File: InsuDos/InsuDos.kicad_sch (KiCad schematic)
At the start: 95 parts, among them J1 E-paper(C097), J2 USB_B_Micro, Q1 Si1308EDL, SW1 list, SW2 enter, SW3 dose, SW4 esc, U1 USBLC6-2P6, U2 TMP102xxDRL, U3 STNS01, U4 STM32WB55CGUx, Y1 32.768k, Y2 32MHz

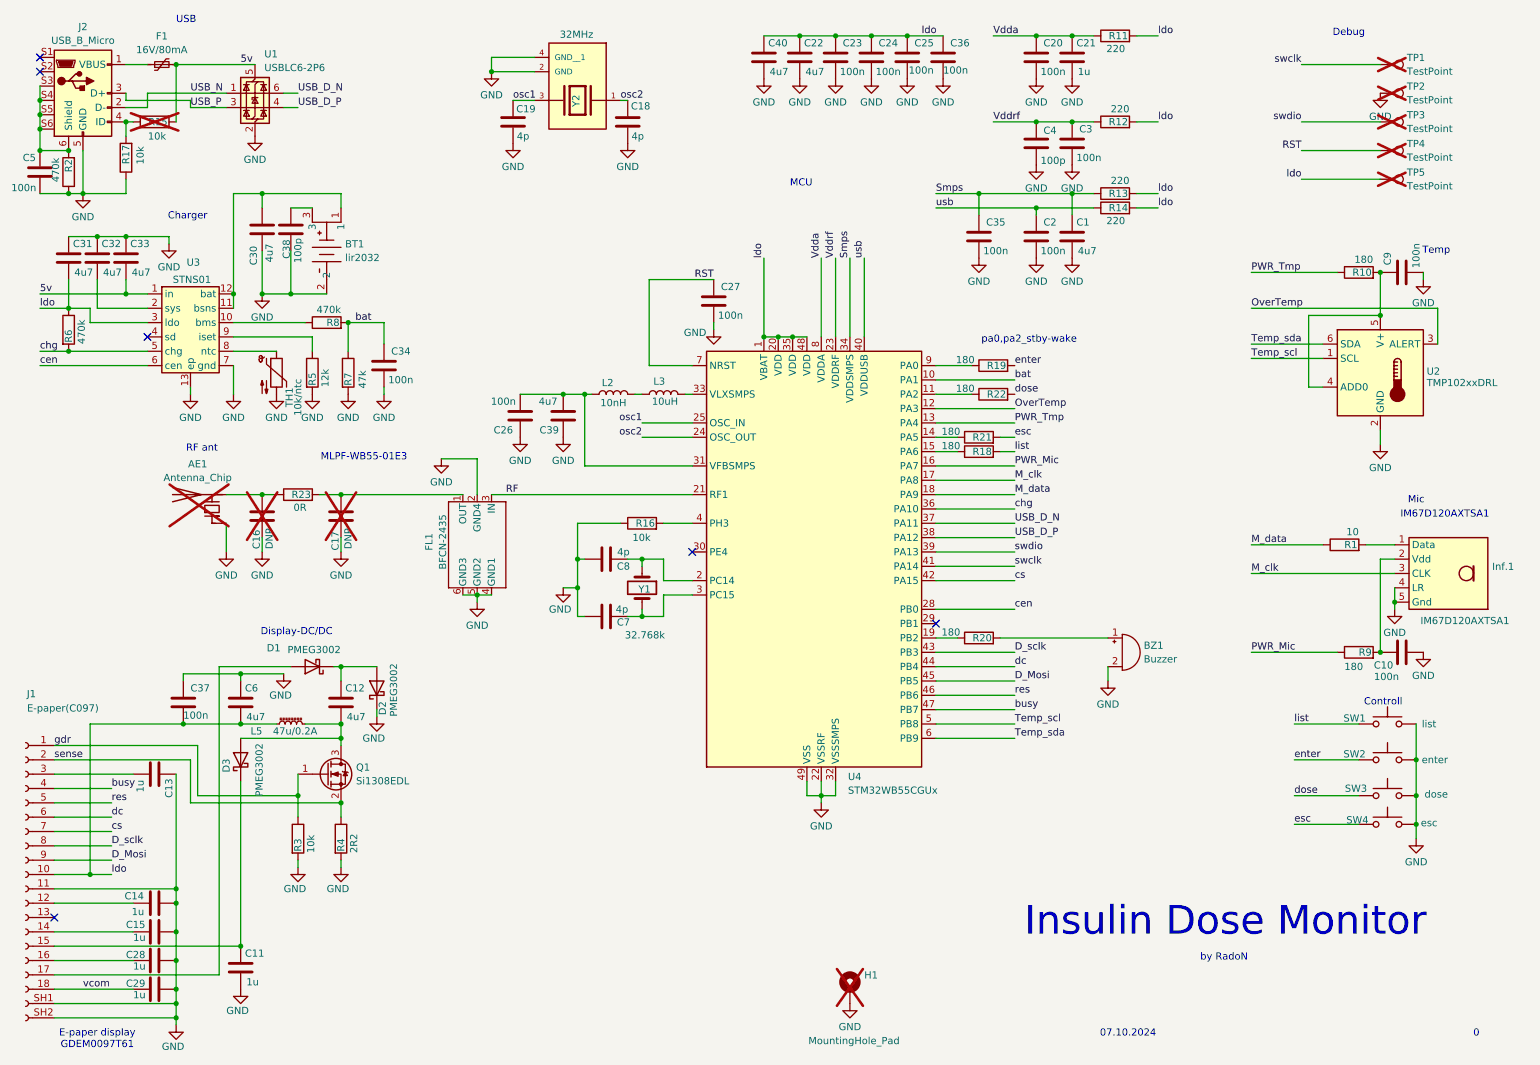
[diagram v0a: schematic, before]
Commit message: added 5v usb detection
pcb not finished, drc missing, 3d models missing, project needs to be cleaned up
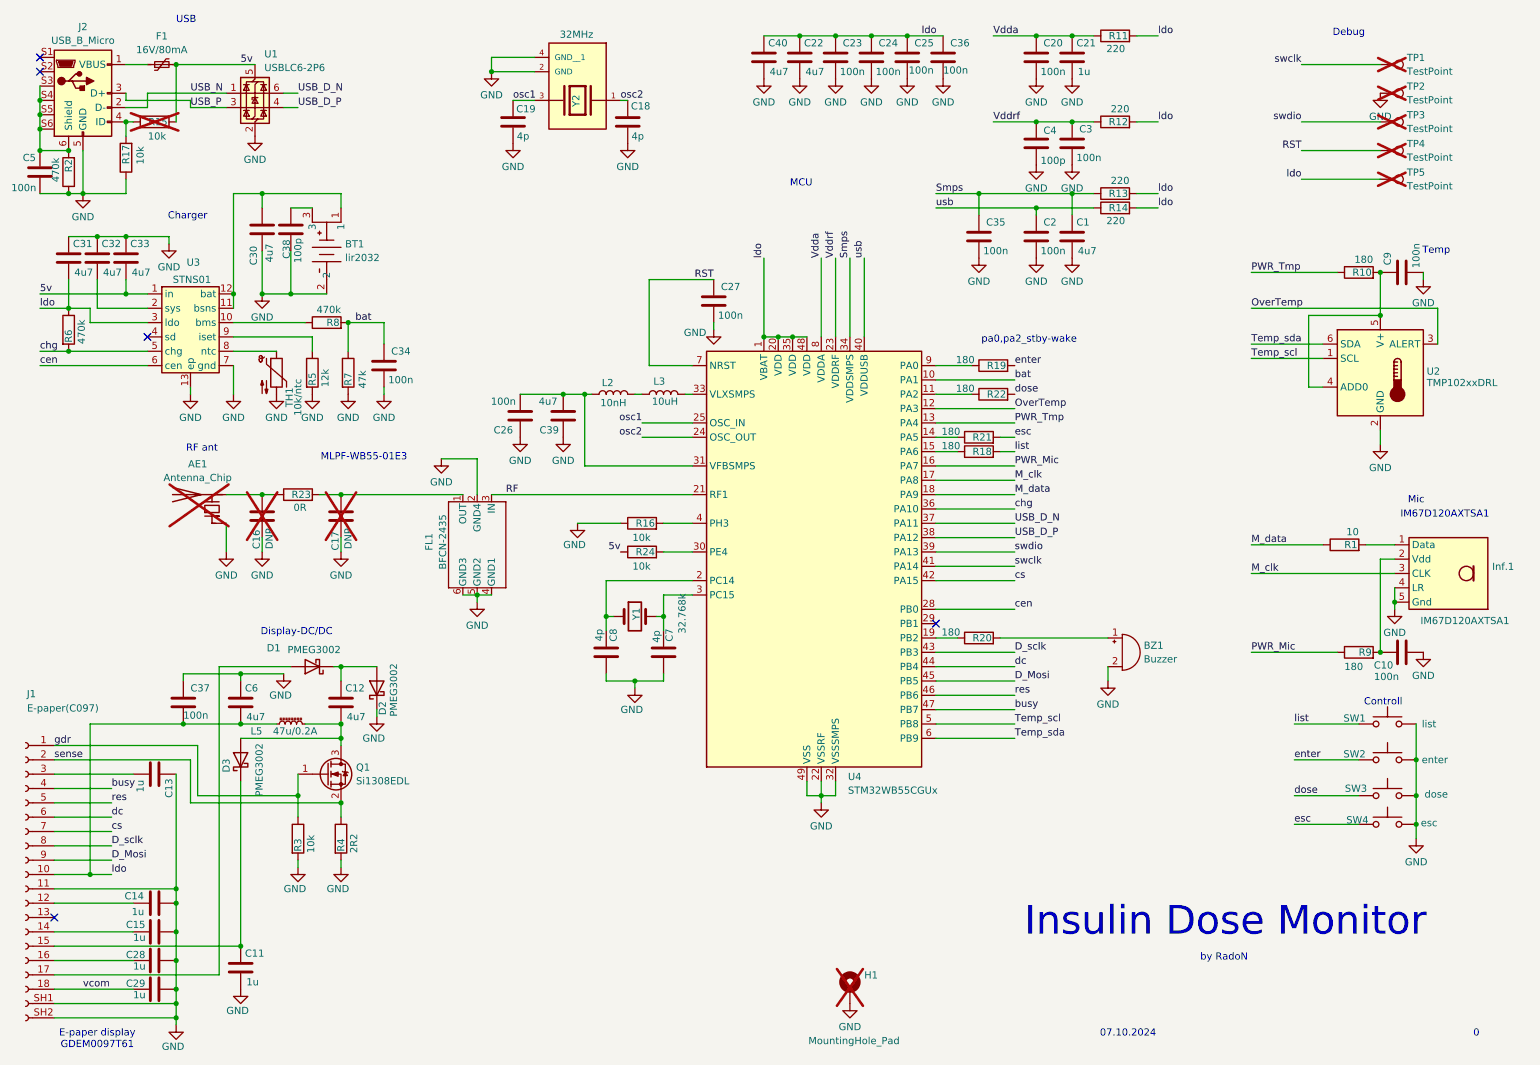
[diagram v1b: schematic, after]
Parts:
- added R24: 10k, Resistor_SMD:R_0402_1005Metric, symbol Device:R
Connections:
- net 5v: now also R24.1
- net at U4.30 (PE4): now also R24.2
- no-connect marks 6 -> 5
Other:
- moved on the sheet: C7, C8, Y1
